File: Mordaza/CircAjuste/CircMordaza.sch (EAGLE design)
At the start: 9 parts, among them IC2 7805TV, X1 SMKDSP_1,5/2

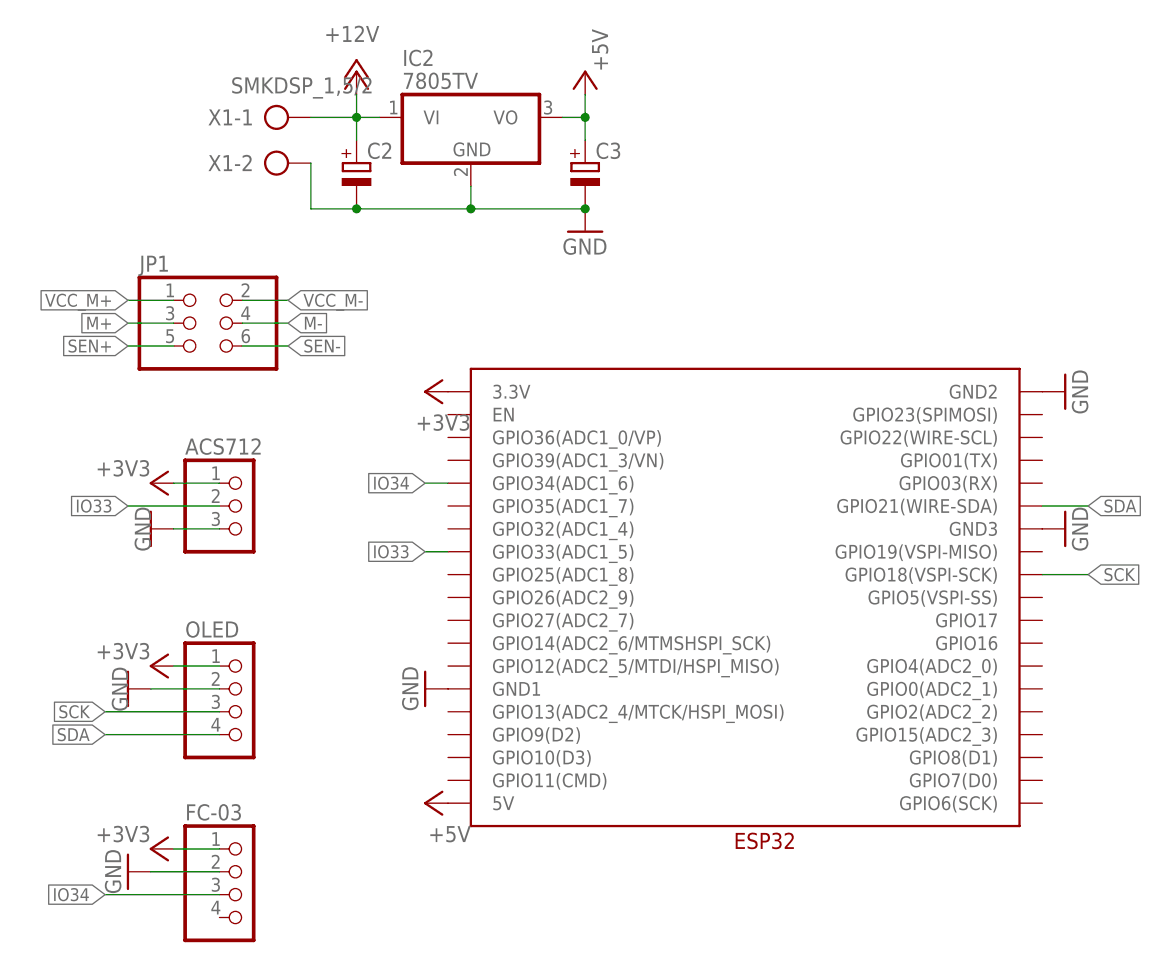
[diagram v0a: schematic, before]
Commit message: Circuito y prog ok 18/06
Circuito y prog ok 18/06
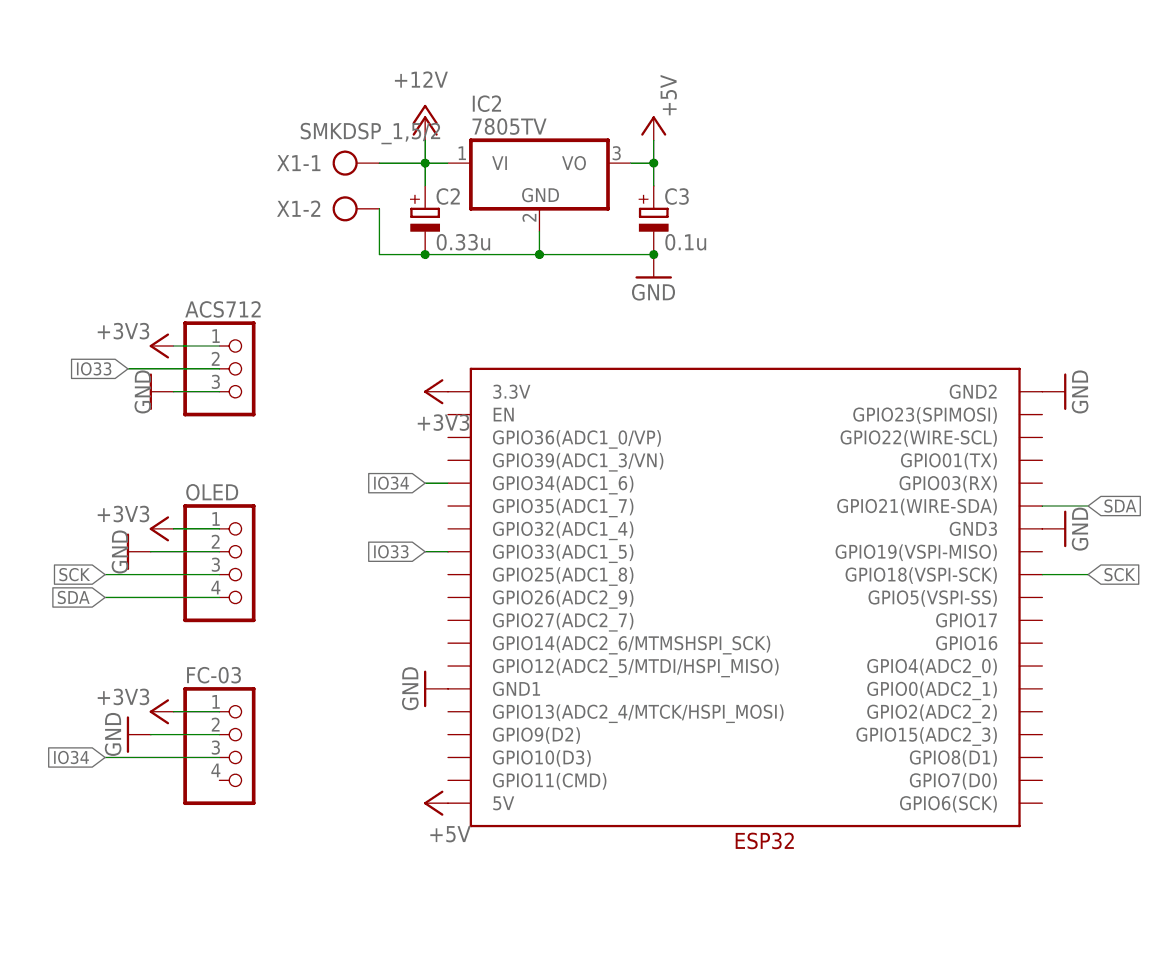
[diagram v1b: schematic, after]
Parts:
- removed JP1: (no value), pinhead:PINHD-2X3
- C2: value (none) -> 0.33u
- C3: value (none) -> 0.1u
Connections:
- removed net M+: JP1.3
- removed net M-: JP1.4
- removed net SEN+: JP1.5
- removed net SEN-: JP1.6
- removed net VCC_M+: JP1.1
- removed net VCC_M-: JP1.2
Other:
- moved on the sheet: ACS712, C2, C3, FC-03, IC2, OLED, X1-1, X1-2
